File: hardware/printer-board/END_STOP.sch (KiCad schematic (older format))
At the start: 18 parts, among them J15 X_MIN, J16 X_MAX, J17 Y_MIN, J18 Y_MAX, J19 Z_MIN, J20 Z_MAX

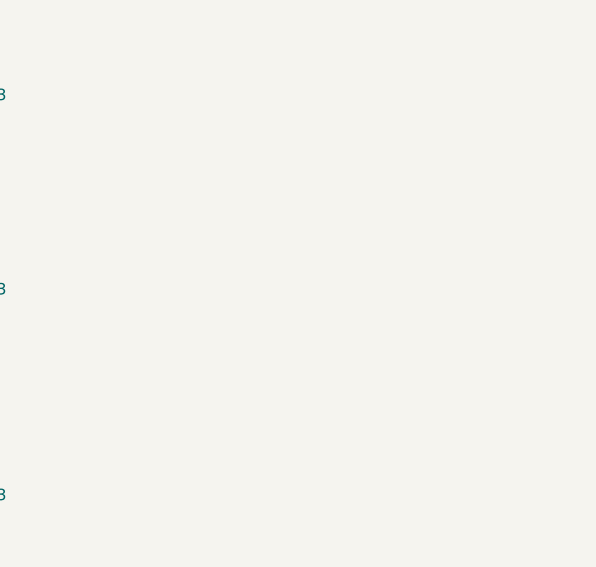
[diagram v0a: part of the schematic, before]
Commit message: update,
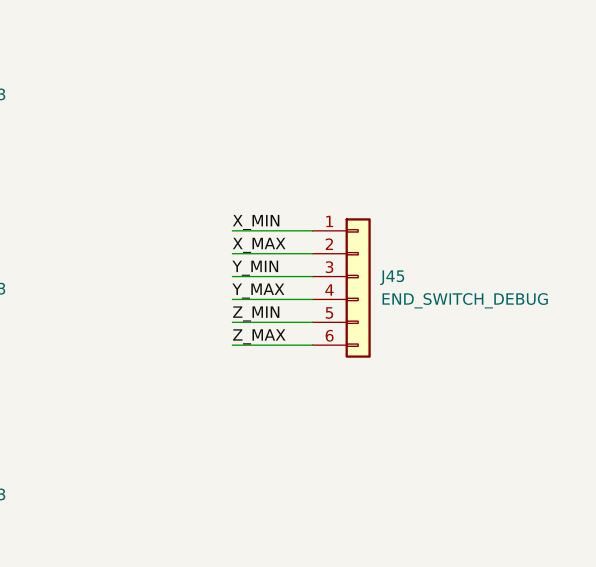
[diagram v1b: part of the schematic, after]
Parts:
- added J45: END_SWITCH_DEBUG, Connector_PinHeader_1.27mm:PinHeader_1x06_P1.27mm_Vertical, symbol Connector_Generic:Conn_01x06
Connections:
- net X_MAX: now also J45.2 (Pin_2)
- net X_MIN: now also J45.1 (Pin_1)
- net Y_MAX: now also J45.4 (Pin_4)
- net Y_MIN: now also J45.3 (Pin_3)
- net Z_MAX: now also J45.6 (Pin_6)
- net Z_MIN: now also J45.5 (Pin_5)
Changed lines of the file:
@@
 Wire Wire Line
 	3800 6600 3800 7250
+$Comp
+L Connector_Generic:Conn_01x06 J45
+U 1 1 5CD1988B
+P 6400 5650
+F 0 "J45" H 6500 5650 50  0000 L CNN
+F 1 "END_SWITCH_DEBUG" H 6500 5550 50  0000 L CNN
+F 2 "Connector_PinHeader_1.27mm:PinHeader_1x06_P1.27mm_Vertical" H 6400 5650 50  0001 C CNN
+F 3 "~" H 6400 5650 50  0001 C CNN
+	1    6400 5650
+	1    0    0    -1
+$EndComp
+Text Label 5850 5450 0    50   ~ 0
+X_MIN
+Text Label 5850 5550 0    50   ~ 0
+X_MAX
+Text Label 5850 5650 0    50   ~ 0
+Y_MIN
+Text Label 5850 5750 0    50   ~ 0
+Y_MAX
+Text Label 5850 5850 0    50   ~ 0
+Z_MIN
+Text Label 5850 5950 0    50   ~ 0
+Z_MAX
+Wire Wire Line
+	5850 5450 6200 5450
+Wire Wire Line
+	5850 5550 6200 5550
+Wire Wire Line
+	5850 5650 6200 5650
+Wire Wire Line
+	5850 5750 6200 5750
+Wire Wire Line
+	5850 5850 6200 5850
+Wire Wire Line
+	5850 5950 6200 5950
 $EndSCHEMATC
